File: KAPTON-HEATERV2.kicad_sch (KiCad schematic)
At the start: 17 parts, among them J1 XT60PW-M, J2 XT60PW-M, J3 1985276, J4 1985218, J5 10090926-P154XLF, K1 1-1393210-8, Q1 AO3400A, U1 TC4427ACOA

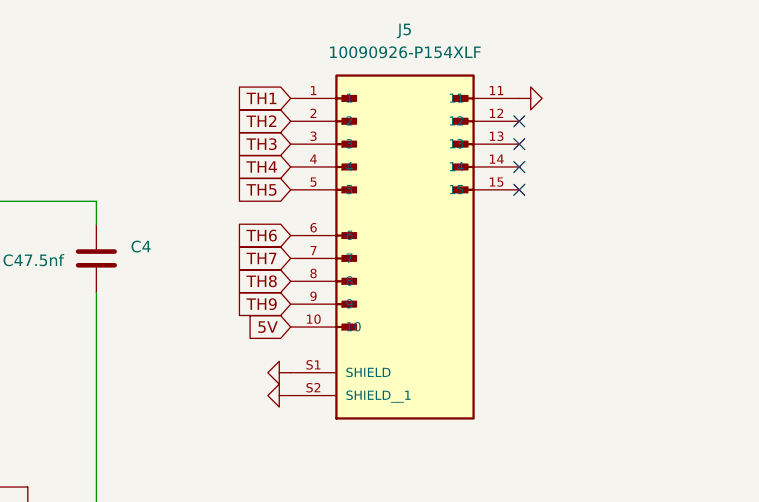
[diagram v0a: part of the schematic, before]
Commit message: forgot to save sch
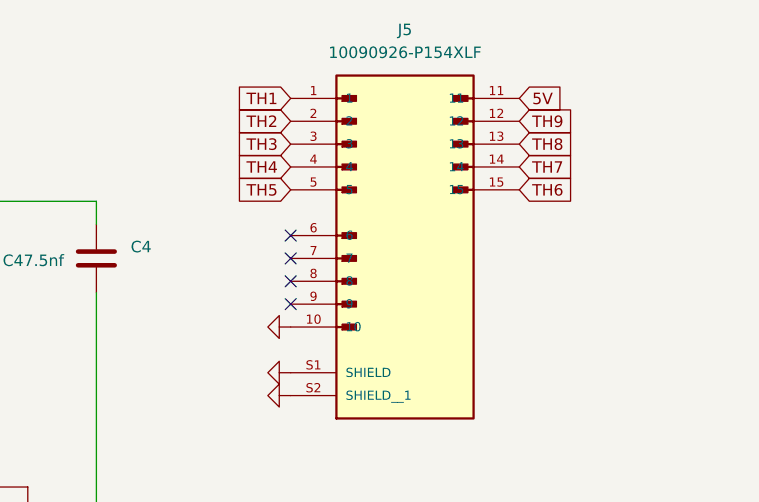
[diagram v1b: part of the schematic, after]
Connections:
- net 5V: now also J5.11; no longer J5.10
- net GND: now also J5.10; no longer J5.11
- net TH6: now also J5.15; no longer J5.6
- net TH7: now also J5.14; no longer J5.7
- net TH8: now also J5.13; no longer J5.8
- net TH9: now also J5.12; no longer J5.9
